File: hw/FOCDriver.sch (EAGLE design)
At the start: 108 parts, among them Q1 BC817, Q2 BC817, Q3 BC817, Q4 BC817, Q5 BC817, Q6 BC817, U1 IRF9389TRPBF, U2 IRF9389TRPBF, U3 LM27313XMF, U4 IRF9389TRPBF, U5 LM358N, U6 LM358N

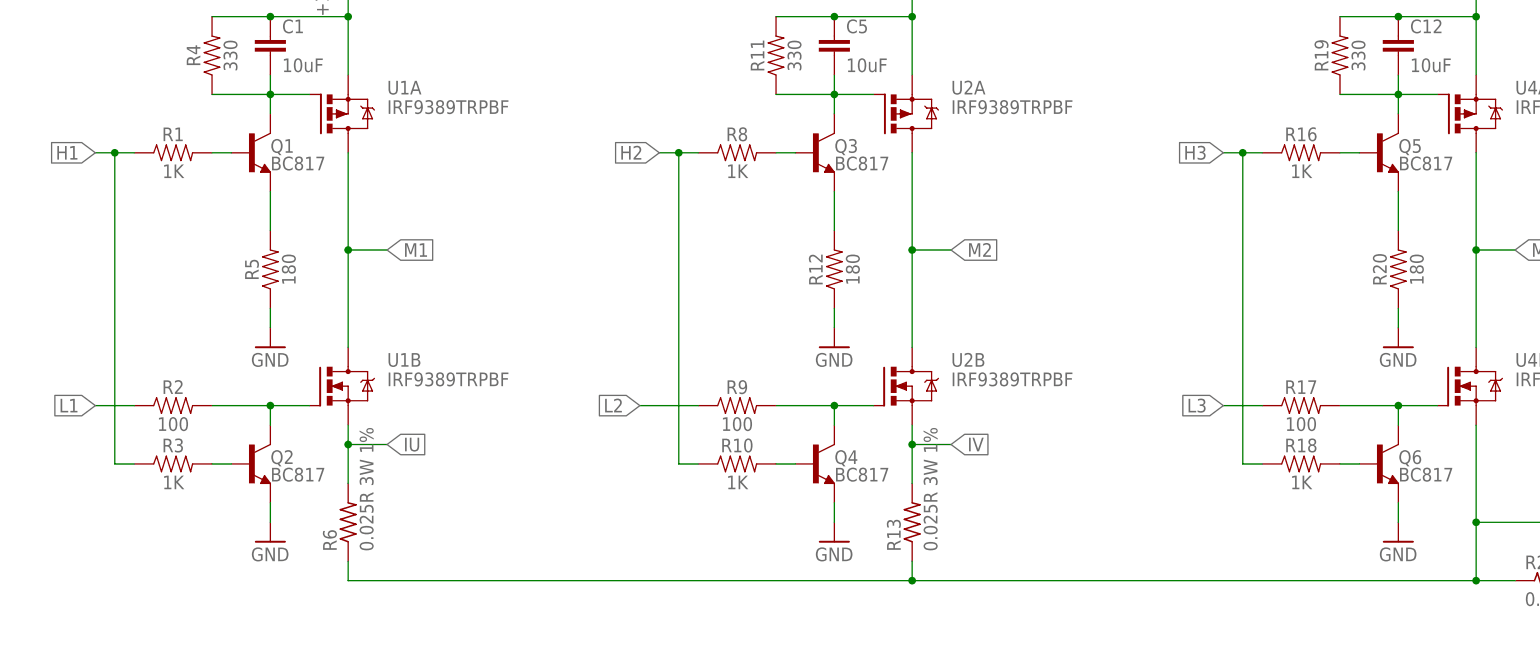
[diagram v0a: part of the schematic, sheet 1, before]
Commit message: simulation
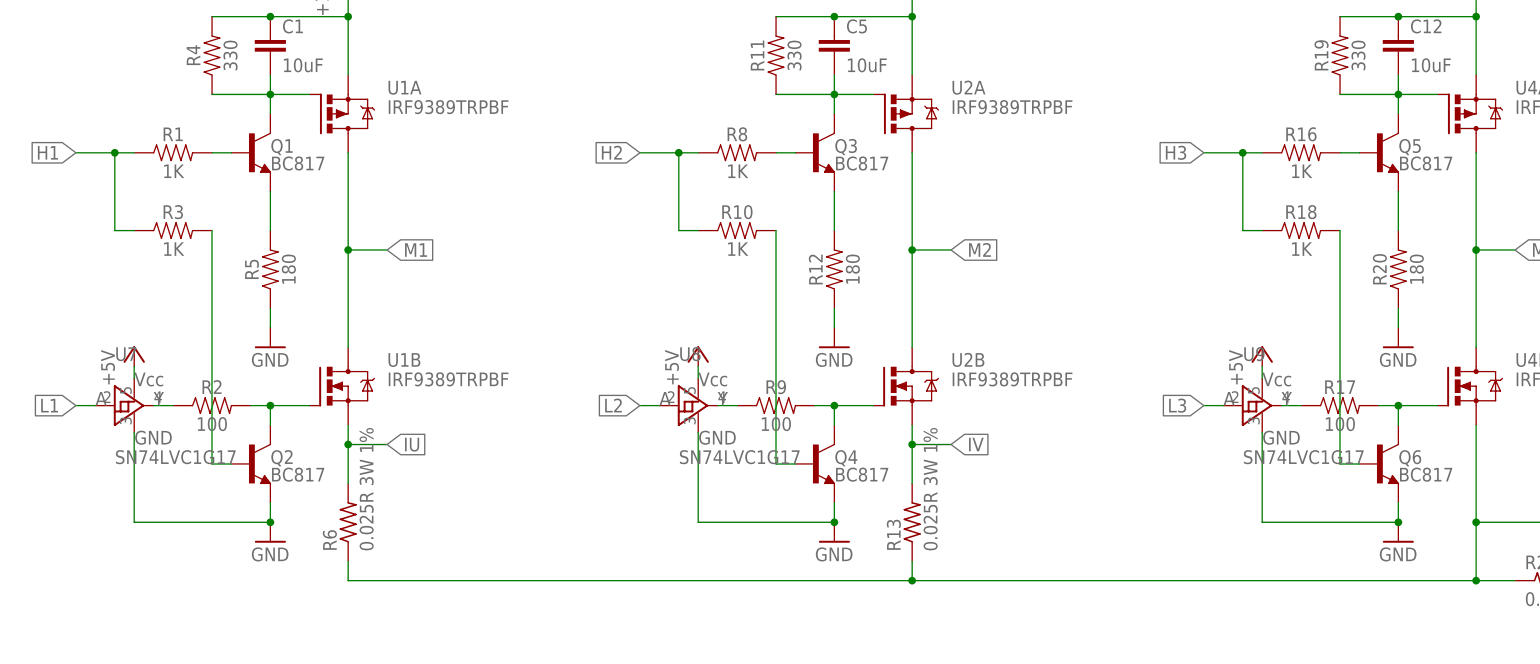
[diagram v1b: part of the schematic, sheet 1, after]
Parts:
- added U7, U8, U9: SN74LVC1G17, SN74LVC1G17:SN74LVC1G17
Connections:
- new net N$46: R2.1, U7.Y
- new net N$47: R9.1, U8.Y
- new net N$48: R17.1, U9.Y
- net +5V: now also U7.VCC, U8.VCC, U9.VCC
- net GND: now also U7.GND, U8.GND, U9.GND
- net L1: now also U7.A; no longer R2.1
- net L2: now also U8.A; no longer R9.1
- net L3: now also U9.A; no longer R17.1
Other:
- moved on the sheet: R10, R17, R18, R2, R3, R9
